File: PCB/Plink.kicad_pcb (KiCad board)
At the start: 2 copper layers, 30 x 30 mm, 39 parts, among them IC1 TLV75533PDBV, J1 USB_B_Mini, J2 STDC14, J3 Target STDC14, J4 I2C_OLED, U1 USBLC6-2SC6, U2 STM32F070CBTx, X1 NX3225GD, X2 Narwahl

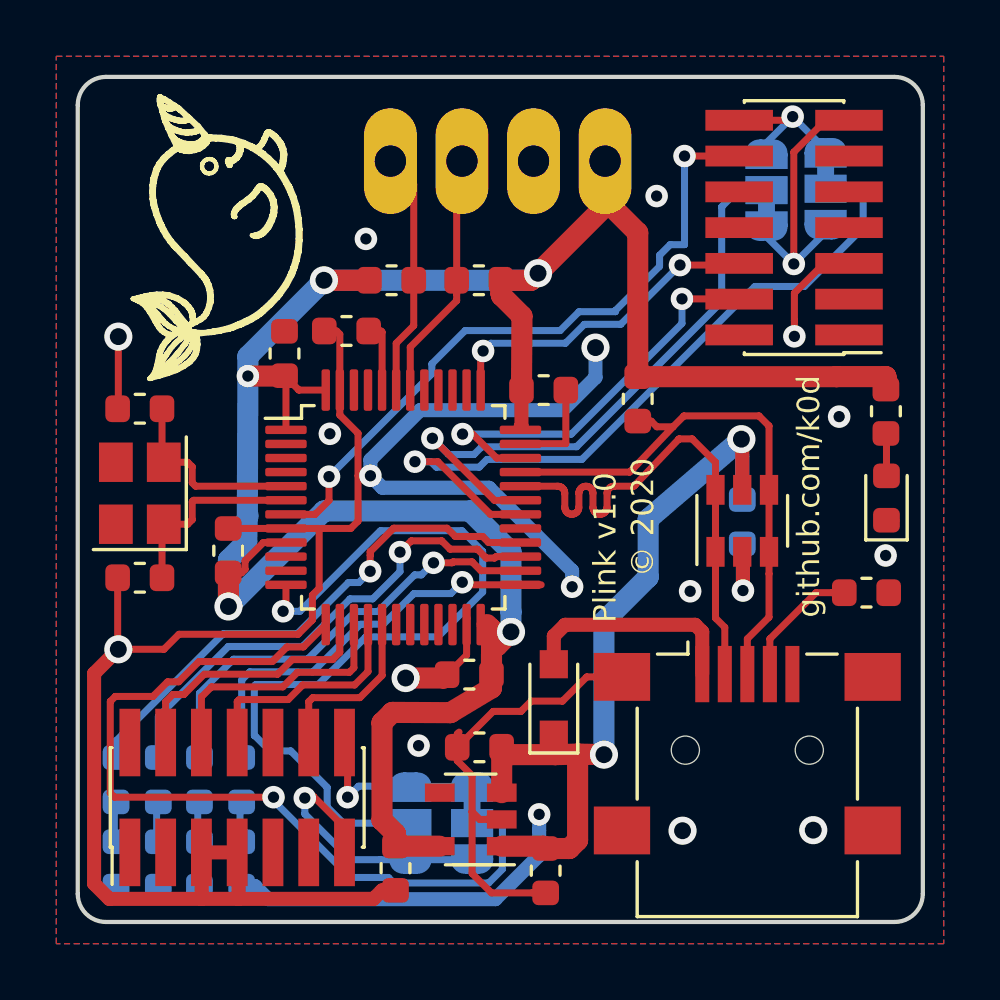
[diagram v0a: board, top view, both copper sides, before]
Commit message: v1.1
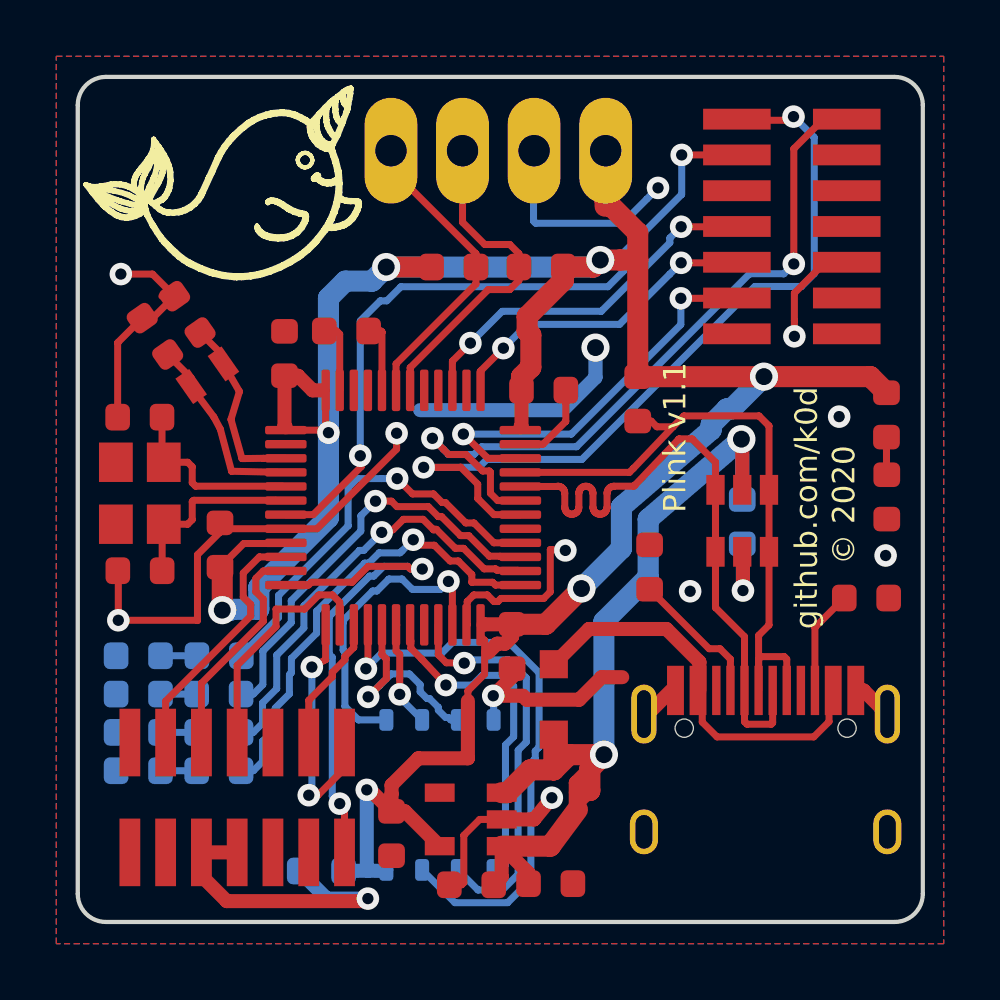
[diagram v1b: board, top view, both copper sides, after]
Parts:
- removed the C2 at (42.5, 45.3)
- removed the J4 at (56.7, 22.4)
- removed JP1: SB_T_VCP_RX, Jumper:SolderJumper-3_P1.3mm_Bridged12_RoundedPad1.0x1.5mm
- removed JP2: SB_T_VCP_TX, Jumper:SolderJumper-3_P1.3mm_Bridged12_RoundedPad1.0x1.5mm
- removed JP3, JP4: SB_VCP_RX, Jumper:SolderJumper-3_P1.3mm_Bridged12_RoundedPad1.0x1.5mm
- removed the R2 at (42.4, 28.7)
- removed the R5 at (56.9, 33.4)
- removed the U2 at (39.8, 36.8)
- added C3: 100nF, 01_Passives:C_0603, F.Cu at (45.0, 50.1)
- added C5: 1uF, 01_Passives:C_0603, F.Cu at (42.2, 50.2)
- added C6: 3.9pF, 01_Passives:C_0603, F.Cu at (32.1, 29.9)
- added C7: 3.9pF, 01_Passives:C_0603, F.Cu at (30.9, 30.7)
- added J3: STDC14, 01_Headers_1.27:M_2x07_1.27_V_SMD, F.Cu at (53.5, 26.8)
- added R11: 5k1, 01_Passives:R_0603, F.Cu at (56.2, 40.0)
- added R4: 4.7k, 01_Passives:R_0603, F.Cu at (41.5, 28.2)
- added R6: 330, 01_Passives:R_0603, F.Cu at (56.9, 33.5)
- added U1: W25Q128JVPIM TR, 01_Packages:WSON_8_6x5_1.27, B.Cu at (41.1, 47.0)
- added U3: STM32L433CCT6, 01_Packages:LQFP_48_7x7_0.5, F.Cu at (39.8, 36.8)
- added X3: 32.768KHz 12.5pF, 01_Packages:Crystal_2p_2012, F.Cu at (32.8, 32.1)
- C1: footprint Capacitor_SMD:C_0603_1608Metric -> 01_Passives:C_0603
- C10: renamed from C8; footprint Capacitor_SMD:C_0603_1608Metric -> 01_Passives:C_0603
- C11: renamed from C9; footprint Capacitor_SMD:C_0603_1608Metric -> 01_Passives:C_0603
- C12: renamed from C10; footprint Capacitor_SMD:C_0603_1608Metric -> 01_Passives:C_0603
- C13: renamed from C11; footprint Capacitor_SMD:C_0603_1608Metric -> 01_Passives:C_0603
- C2: renamed from C3; footprint Capacitor_SMD:C_0603_1608Metric -> 01_Passives:C_0603
- C4: value 1uF -> 100nF; footprint Capacitor_SMD:C_0603_1608Metric -> 01_Passives:C_0603; moved to B.Cu
- C8: renamed from C6; footprint Capacitor_SMD:C_0603_1608Metric -> 01_Passives:C_0603
- C9: renamed from C5; footprint Capacitor_SMD:C_0603_1608Metric -> 01_Passives:C_0603
- D1: footprint Diode_SMD:D_SOD-323_HandSoldering -> 01_Passives:D_SOD_323
- D2, D3, D4, D5, D6: footprint LED_SMD:LED_0603_1608Metric -> 01_Passives:LED_0603
- IC1: footprint Package_TO_SOT_SMD:SOT-23-5 -> 01_Packages:SOT-23-5
- J1: value USB_B_Mini -> USB_C_Socket_USB2.0; footprint Connector_USB:USB_Mini-B_Lumberg_2486_01_Horizontal -> 01_Connectors:USB_C_Socket-C319148
- J2: value STDC14 -> I2C_OLED; footprint Connector_PinHeader_1.27mm:PinHeader_2x07_P1.27mm_Vertical_SMD -> 00_Components:OLED_i2c; moved to B.Cu
- J4: renamed from J3; footprint Connector_PinHeader_1.27mm:PinHeader_2x07_P1.27mm_Vertical_SMD -> 01_Headers_1.27:M_2x07_1.27_V_SMD
- R1, R3: footprint Resistor_SMD:R_0603_1608Metric -> 01_Passives:R_0603
- R10: renamed from R9; footprint Resistor_SMD:R_0603_1608Metric -> 01_Passives:R_0603
- R2: renamed from R10; value 100k -> 5k1; footprint Resistor_SMD:R_0603_1608Metric -> 01_Passives:R_0603
- R5: renamed from R4; footprint Resistor_SMD:R_0603_1608Metric -> 01_Passives:R_0603
- R7: renamed from R6; footprint Resistor_SMD:R_0603_1608Metric -> 01_Passives:R_0603
- R8: renamed from R7; footprint Resistor_SMD:R_0603_1608Metric -> 01_Passives:R_0603
- R9: renamed from R8; footprint Resistor_SMD:R_0603_1608Metric -> 01_Passives:R_0603
- U2: renamed from U1; footprint Package_TO_SOT_SMD:SOT-23-6 -> 01_Packages:SOT-23-6
- X2: renamed from X1; value NX3225GD -> 8MHz 8pF; footprint Crystal:Crystal_SMD_3225-4Pin_3.2x2.5mm -> 01_Packages:Crystal_4p_3225
- moved C4 7.96 mm to (36.9, 49.7), turned to 0 degrees
- moved R2 7.75 mm to (48.5, 38.9), turned to 270 degrees
- moved D6 7.43 mm to (30.4, 42.0), turned to 0 degrees
- moved D5 6.07 mm to (30.4, 43.4), turned to 0 degrees
- moved J2 5.75 mm to (56.7, 22.0)
- moved R10 5.72 mm to (33.2, 42.0), turned to 180 degrees
- moved R3 5.33 mm to (44.6, 28.2), turned to 0 degrees
- moved D4 5.15 mm to (30.4, 44.8), turned to 0 degrees
- moved D3 4.94 mm to (30.4, 46.1), turned to 0 degrees
- moved R9 3.72 mm to (33.2, 43.4), turned to 180 degrees
- moved X1 2.47 mm to (33.5, 25.2), turned to 357 degrees
- moved C10 1.82 mm to (43.6, 41.7), turned to 90 degrees
- moved R8 1.82 mm to (33.2, 44.8), turned to 180 degrees
- moved C8 1.24 mm to (39.3, 48.4)
- moved J1 1.22 mm to (52.6, 46.4)
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- renumbered X2 to X1
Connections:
- C4 pad 2: +5V -> +3V3
- J2 pad 1: Net-(J2-Pad1) -> +3V3
- J2 pad 2: Net-(J2-Pad2) -> GND
- J2 pad 3: Net-(J2-Pad3) -> /I2C1_SCL
- J2 pad 4: /DBG_DIO -> /I2C1_SDA
- J4 pad 13: /PIN_T_VCP_RX -> /T_VCP_RX
- J4 pad 14: /PIN_T_VCP_TX -> /T_VCP_TX
- J4 pad 4: /T_DBG_DIO -> /T_SWDIO
- J4 pad 6: /T_DBG_CLK -> /T_SWCLK
- J4 pad 8: /T_DBG_SWO -> /T_SWO
- R2 pad 1: Net-(J1-Pad4) -> GND
- R2 pad 2: GND -> Net-(J1-PadA5)
- R3 pad 1: /I2C1_SDA -> /I2C1_SCL
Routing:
- net GND: track 116.5 -> 87.2 mm, vias 18 -> 14
- net /T_VCP_TX: track 30.2 -> 8.98 mm, vias 1 -> 2
- net /FLASH_D3: track 0.00 -> 20.8 mm, vias 0 -> 1
- net /DBG_DIO: track 14.7 -> 0.00 mm, vias 2 -> 0
- net /SWDIO: track 0.00 -> 14.6 mm, vias 0 -> 2
- net /FLASH_CLK: track 0.00 -> 14.4 mm, vias 0 -> 1
- net /SWO: track 0.00 -> 13.2 mm, vias 0 -> 2
- net /FLASH_D0: track 0.00 -> 12.3 mm, vias 0 -> 1
- net /DBG_CLK: track 11.8 -> 0.00 mm, vias 2 -> 0
- net /PIN_T_VCP_RX: track 11.8 -> 0.00 mm, vias 1 -> 0
- net /T_VCP_RX: track 29.5 -> 17.8 mm, vias 1 -> 2
- net /SWCLK: track 0.00 -> 11.5 mm, vias 0 -> 2
- net /FLASH_CS: track 0.00 -> 11.0 mm, vias 0 -> 1
- net /PIN_VCP_RX: track 10.8 -> 0.00 mm, vias 1 -> 0
- net /T_DBG_DIO: track 9.34 -> 0.00 mm
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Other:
- rule pad_to_mask_clearance: 0.07 -> 0
- board text added: "Plink v1.1"
- board text removed: "Plink v1.0"
